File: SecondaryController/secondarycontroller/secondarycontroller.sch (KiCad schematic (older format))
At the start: 11 parts

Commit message: Meh, doesnt work
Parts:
- CF15: footprint (none) -> Capacitor_THT:C_Rect_L41.5mm_W19.0mm_P37.50mm_MKS4; symbol Device:C -> secondarycontroller-rescue:C-Device
- D1, D2: renamed from D?; footprint (none) -> Diode_THT:D_5W_P12.70mm_Horizontal; symbol pspice:DIODE -> secondarycontroller-rescue:DIODE-pspice
- J1: renamed from J?; value Conn_01x03_Female -> Receiver; footprint (none) -> Connector_PinHeader_2.54mm:PinHeader_1x03_P2.54mm_Vertical; symbol Connector:Conn_01x03_Female -> secondarycontroller-rescue:Conn_01x03_Female-Connector
- J3: renamed from J?; value Conn_01x02_Female -> VIN; footprint (none) -> Connector_PinHeader_2.54mm:PinHeader_1x02_P2.54mm_Vertical; symbol Connector:Conn_01x02_Female -> secondarycontroller-rescue:Conn_01x02_Female-Connector
- J4: renamed from J?; footprint (none) -> Connector_PinHeader_2.54mm:PinHeader_1x04_P2.54mm_Vertical; symbol Connector:Conn_01x04_Female -> secondarycontroller-rescue:Conn_01x04_Female-Connector
- J5: renamed from J?; value Conn_01x02_Female -> I2C BUS; footprint (none) -> Connector_PinHeader_2.54mm:PinHeader_1x02_P2.54mm_Vertical; symbol Connector:Conn_01x02_Female -> secondarycontroller-rescue:Conn_01x02_Female-Connector
- SW1: renamed from Calibrate; value SW_Push -> Calibrate; footprint (none) -> Button_Switch_THT:SW_DIP_SPSTx01_Piano_10.8x4.1mm_W7.62mm_P2.54mm; symbol Switch:SW_Push -> secondarycontroller-rescue:SW_Push-Switch
- SW2: renamed from Reset; value SW_Push -> Reset; footprint (none) -> Button_Switch_THT:SW_DIP_SPSTx01_Piano_10.8x4.1mm_W7.62mm_P2.54mm; symbol Switch:SW_Push -> secondarycontroller-rescue:SW_Push-Switch
- U1: renamed from U?; symbol mcu3386:MCU3386 -> secondarycontroller-rescue:MCU3386-mcu3386
- XA1: renamed from XA?; symbol arduino:Arduino_Uno_Shield -> secondarycontroller-rescue:Arduino_Uno_Shield-arduino
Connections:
- wire segments 73 -> 68
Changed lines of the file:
@@
 EESchema Schematic File Version 4
+LIBS:secondarycontroller-cache
 EELAYER 26 0
 EELAYER END
@@
 $EndDescr
 $Comp
-L arduino:Arduino_Uno_Shield XA?
+L secondarycontroller-rescue:Arduino_Uno_Shield-arduino XA1
 U 1 1 5BBE520D
 P 4100 2750
-F 0 "XA?" H 4100 4137 60  0000 C CNN
+F 0 "XA1" H 4100 4137 60  0000 C CNN
 F 1 "Arduino_Uno_Shield" H 4100 4031 60  0000 C CNN
 F 2 "" H 5900 6500 60  0001 C CNN
@@
 $EndComp
 $Comp
-L Connector:Conn_01x02_Female J?
+L secondarycontroller-rescue:Conn_01x02_Female-Connector J3
 U 1 1 5BBE53F0
 P 1900 3600
-F 0 "J?" H 1794 3275 50  0000 C CNN
-F 1 "Conn_01x02_Female" H 1794 3366 50  0000 C CNN
-F 2 "" H 1900 3600 50  0001 C CNN
+F 0 "J3" H 1794 3275 50  0000 C CNN
+F 1 "VIN" H 1794 3366 50  0000 C CNN
+F 2 "Connector_PinHeader_2.54mm:PinHeader_1x02_P2.54mm_Vertical" H 1900 3600 50  0001 C CNN
 F 3 "~" H 1900 3600 50  0001 C CNN
 	1    1900 3600
@@
 	2550 3300 2800 3300
 $Comp
-L Device:C CF15
+L secondarycontroller-rescue:C-Device CF15
 U 1 1 5BBE583A
 P 2400 4300
 F 0 "CF15" V 2148 4300 50  0000 C CNN
 F 1 "C" V 2239 4300 50  0000 C CNN
-F 2 "" H 2438 4150 50  0001 C CNN
+F 2 "Capacitor_THT:C_Rect_L41.5mm_W19.0mm_P37.50mm_MKS4" H 2438 4150 50  0001 C CNN
 F 3 "~" H 2400 4300 50  0001 C CNN
 	1    2400 4300
@@
 $EndComp
 $Comp
-L pspice:DIODE D?
+L secondarycontroller-rescue:DIODE-pspice D2
 U 1 1 5BBE5A38
 P 2550 5100
-F 0 "D?" V 2596 4972 50  0000 R CNN
+F 0 "D2" V 2596 4972 50  0000 R CNN
 F 1 "DIODE" V 2505 4972 50  0000 R CNN
-F 2 "" H 2550 5100 50  0001 C CNN
+F 2 "Diode_THT:D_5W_P12.70mm_Horizontal" H 2550 5100 50  0001 C CNN
 F 3 "~" H 2550 5100 50  0001 C CNN
 	1    2550 5100
@@
 $EndComp
 $Comp
-L Switch:SW_Push Reset
+L secondarycontroller-rescue:SW_Push-Switch SW2
 U 1 1 5BBE645A
 P 4100 4300
-F 0 "Reset" H 4100 4585 50  0000 C CNN
-F 1 "SW_Push" H 4100 4494 50  0000 C CNN
-F 2 "" H 4100 4500 50  0001 C CNN
+F 0 "SW2" H 4100 4585 50  0000 C CNN
+F 1 "Reset" H 4100 4494 50  0000 C CNN
+F 2 "Button_Switch_THT:SW_DIP_SPSTx01_Piano_10.8x4.1mm_W7.62mm_P2.54mm" H 4100 4500 50  0001 C CNN
 F 3 "" H 4100 4500 50  0001 C CNN
 	1    4100 4300
@@
 $EndComp
 $Comp
-L Connector:Conn_01x04_Female J?
+L secondarycontroller-rescue:Conn_01x04_Female-Connector J4
 U 1 1 5BBE6815
 P 6250 1600
-F 0 "J?" H 6278 1576 50  0000 L CNN
+F 0 "J4" H 6278 1576 50  0000 L CNN
 F 1 "APA102C" H 6278 1485 50  0000 L CNN
-F 2 "" H 6250 1600 50  0001 C CNN
+F 2 "Connector_PinHeader_2.54mm:PinHeader_1x04_P2.54mm_Vertical" H 6250 1600 50  0001 C CNN
 F 3 "~" H 6250 1600 50  0001 C CNN
 	1    6250 1600
@@
 $EndComp
 $Comp
-L Switch:SW_Push Calibrate
+L secondarycontroller-rescue:SW_Push-Switch SW1
 U 1 1 5BBE694D
-P 7100 2050
-F 0 "Calibrate" H 7100 2335 50  0000 C CNN
-F 1 "SW_Push" H 7100 2244 50  0000 C CNN
-F 2 "" H 7100 2250 50  0001 C CNN
-F 3 "" H 7100 2250 50  0001 C CNN
-	1    7100 2050
+P 5600 2100
+F 0 "SW1" H 5600 2385 50  0000 C CNN
+F 1 "Calibrate" H 5600 2294 50  0000 C CNN
+F 2 "Button_Switch_THT:SW_DIP_SPSTx01_Piano_10.8x4.1mm_W7.62mm_P2.54mm" H 5600 2300 50  0001 C CNN
+F 3 "" H 5600 2300 50  0001 C CNN
+	1    5600 2100
 	1    0    0    -1
 $EndComp
@@
 Connection ~ 2550 3600
 $Comp
-L mcu3386:MCU3386 U?
+L secondarycontroller-rescue:MCU3386-mcu3386 U1
 U 1 1 5BBE76D9
 P 1300 4750
-F 0 "U?" H 1350 4865 50  0000 C CNN
+F 0 "U1" H 1350 4865 50  0000 C CNN
 F 1 "MCU3386" H 1350 4774 50  0000 C CNN
 F 2 "" H 1300 4750 50  0001 C CNN
@@
 	2550 4300 2550 3600
 $Comp
-L pspice:DIODE D?
+L secondarycontroller-rescue:DIODE-pspice D1
 U 1 1 5BBE875F
 P 2200 5200
-F 0 "D?" H 2200 4935 50  0000 C CNN
+F 0 "D1" H 2200 4935 50  0000 C CNN
 F 1 "DIODE" H 2200 5026 50  0000 C CNN
-F 2 "" H 2200 5200 50  0001 C CNN
+F 2 "Diode_THT:D_5W_P12.70mm_Horizontal" H 2200 5200 50  0001 C CNN
 F 3 "~" H 2200 5200 50  0001 C CNN
 	1    2200 5200
@@
 	1550 4300 2250 4300
 $Comp
-L Connector:Conn_01x03_Female J?
+L secondarycontroller-rescue:Conn_01x03_Female-Connector J1
 U 1 1 5BBEDF33
 P 6200 2300
-F 0 "J?" H 6227 2326 50  0000 L CNN
-F 1 "Conn_01x03_Female" H 6227 2235 50  0000 L CNN
-F 2 "" H 6200 2300 50  0001 C CNN
+F 0 "J1" H 6227 2326 50  0000 L CNN
+F 1 "Receiver" H 6227 2235 50  0000 L CNN
+F 2 "Connector_PinHeader_2.54mm:PinHeader_1x03_P2.54mm_Vertical" H 6200 2300 50  0001 C CNN
 F 3 "~" H 6200 2300 50  0001 C CNN
 	1    6200 2300
@@
 Connection ~ 2900 5400
 Wire Wire Line
-	5400 2100 5800 2100
-Wire Wire Line
-	5800 2100 5800 1950
-Wire Wire Line
-	5800 1950 6900 1950
-Wire Wire Line
-	6900 1950 6900 2050
-Wire Wire Line
-	7300 2050 7300 1400
-Wire Wire Line
-	7300 1400 5850 1400
-Wire Wire Line
-	5850 1400 5850 1500
-Connection ~ 5850 1500
+	5800 2100 5850 2100
+Wire Wire Line
+	5850 2100 5850 2050
 Wire Wire Line
 	5850 1500 5850 2050
 $Comp
-L Connector:Conn_01x02_Female J?
+L secondarycontroller-rescue:Conn_01x02_Female-Connector J5
 U 1 1 5BBF72BA
 P 2300 2100
-F 0 "J?" H 2194 1775 50  0000 C CNN
-F 1 "Conn_01x02_Female" H 2194 1866 50  0000 C CNN
-F 2 "" H 2300 2100 50  0001 C CNN
+F 0 "J5" H 2194 1775 50  0000 C CNN
+F 1 "I2C BUS" H 2194 1866 50  0000 C CNN
+F 2 "Connector_PinHeader_2.54mm:PinHeader_1x02_P2.54mm_Vertical" H 2300 2100 50  0001 C CNN
 F 3 "~" H 2300 2100 50  0001 C CNN
 	1    2300 2100
@@
 Wire Wire Line
 	2500 2100 2800 2100
+Connection ~ 5850 2050
 $EndSCHEMATC

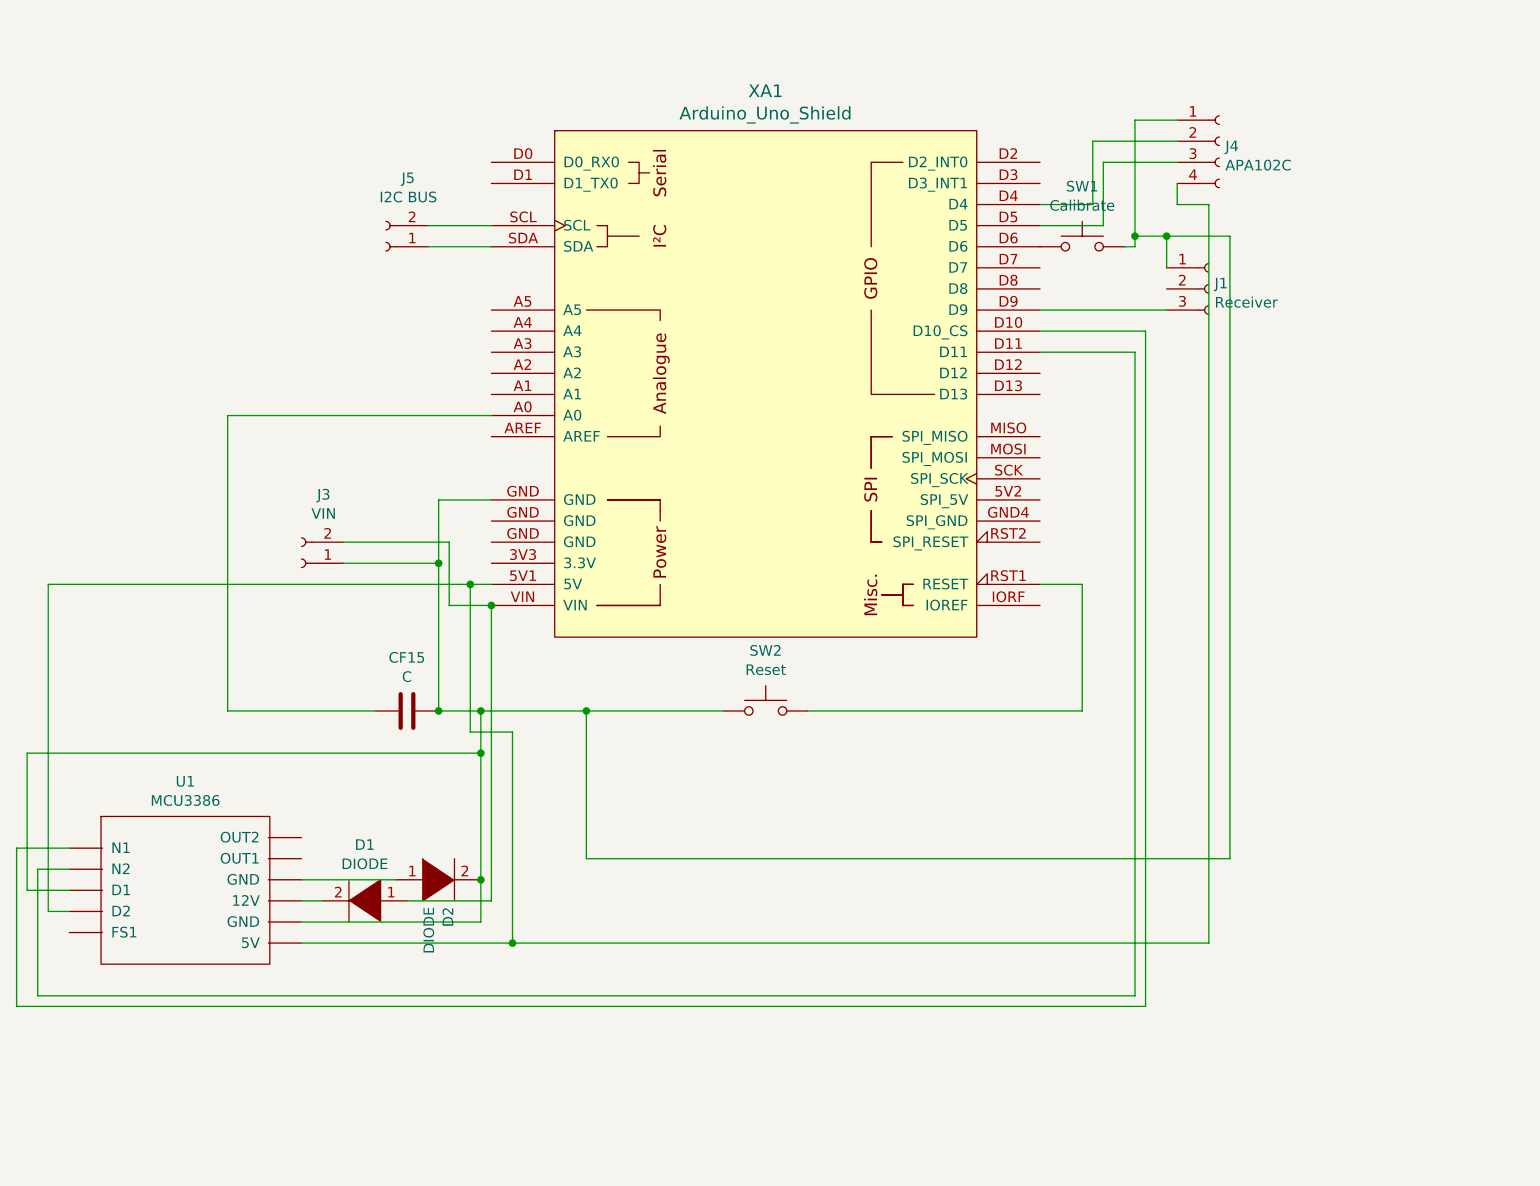
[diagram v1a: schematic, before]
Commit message: Finished PCB Secondary
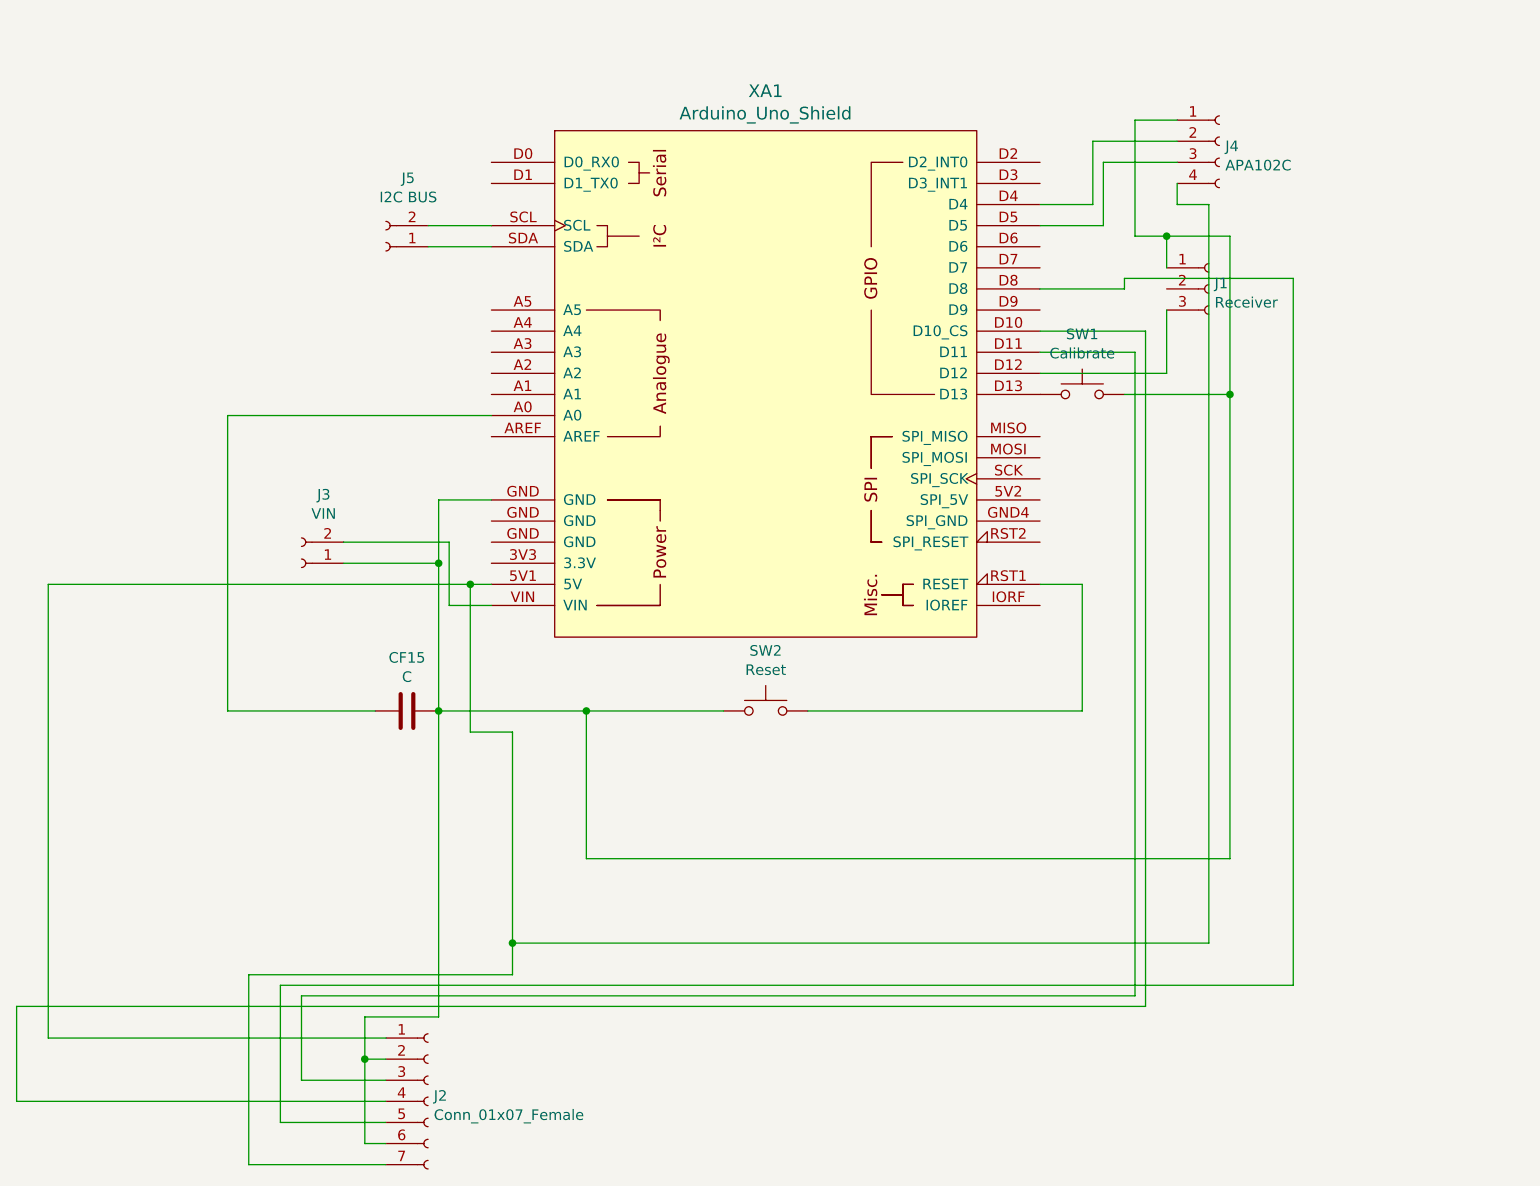
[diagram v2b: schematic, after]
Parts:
- removed D1, D2: DIODE, Diode_THT:D_5W_P12.70mm_Horizontal, symbol secondarycontroller-rescue:DIODE-pspice
- removed U1: MCU3386, symbol secondarycontroller-rescue:MCU3386-mcu3386
- added J2: Conn_01x07_Female, Connector_PinSocket_2.54mm:PinSocket_1x07_P2.54mm_Vertical, symbol Connector:Conn_01x07_Female
- CF15: footprint Capacitor_THT:C_Rect_L41.5mm_W19.0mm_P37.50mm_MKS4 -> Capacitor_THT:C_Rect_L41.5mm_W13.0mm_P37.50mm_MKS4
- SW1, SW2: footprint Button_Switch_THT:SW_DIP_SPSTx01_Piano_10.8x4.1mm_W7.62mm_P2.54mm -> Button_Switch_THT:SW_PUSH_6mm
- XA1: footprint (none) -> Arduino:Arduino_Uno_Shield
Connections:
- net at J4.4 (Pin_4), XA1.5V1 (5V): now also J2.1 (Pin_1), J2.7 (Pin_7)
- net at XA1.D10 (D10_CS): now also J2.4 (Pin_4)
- net at XA1.D11: now also J2.3 (Pin_3)
- net at XA1.D12: now also J1.3 (Pin_3)
- net at XA1.D13: now also SW1.1
- net at XA1.D6: no longer SW1.1
- net at XA1.D8: now also J2.5 (Pin_5)
- net at XA1.D9: no longer J1.3 (Pin_3)
- net at XA1.GND: now also CF15.1, J1.1 (Pin_1), J3.1 (Pin_1), J4.1 (Pin_1), SW1.2, SW2.1, J2.2 (Pin_2), J2.6 (Pin_6)
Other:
- moved on the sheet: SW1
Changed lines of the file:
@@
 F 0 "XA1" H 4100 4137 60  0000 C CNN
 F 1 "Arduino_Uno_Shield" H 4100 4031 60  0000 C CNN
-F 2 "" H 5900 6500 60  0001 C CNN
+F 2 "Arduino:Arduino_Uno_Shield" H 5900 6500 60  0001 C CNN
 F 3 "https://store.arduino.cc/arduino-uno-rev3" H 5900 6500 60  0001 C CNN
 	1    4100 2750
@@
 F 0 "CF15" V 2148 4300 50  0000 C CNN
 F 1 "C" V 2239 4300 50  0000 C CNN
-F 2 "Capacitor_THT:C_Rect_L41.5mm_W19.0mm_P37.50mm_MKS4" H 2438 4150 50  0001 C CNN
+F 2 "Capacitor_THT:C_Rect_L41.5mm_W13.0mm_P37.50mm_MKS4" H 2438 4150 50  0001 C CNN
 F 3 "~" H 2400 4300 50  0001 C CNN
 	1    2400 4300
 	0    1    1    0
-$EndComp
-$Comp
-L secondarycontroller-rescue:DIODE-pspice D2
-U 1 1 5BBE5A38
-P 2550 5100
-F 0 "D2" V 2596 4972 50  0000 R CNN
-F 1 "DIODE" V 2505 4972 50  0000 R CNN
-F 2 "Diode_THT:D_5W_P12.70mm_Horizontal" H 2550 5100 50  0001 C CNN
-F 3 "~" H 2550 5100 50  0001 C CNN
-	1    2550 5100
-	1    0    0    -1
 $EndComp
 $Comp
@@
 F 0 "SW2" H 4100 4585 50  0000 C CNN
 F 1 "Reset" H 4100 4494 50  0000 C CNN
-F 2 "Button_Switch_THT:SW_DIP_SPSTx01_Piano_10.8x4.1mm_W7.62mm_P2.54mm" H 4100 4500 50  0001 C CNN
+F 2 "Button_Switch_THT:SW_PUSH_6mm" H 4100 4500 50  0001 C CNN
 F 3 "" H 4100 4500 50  0001 C CNN
 	1    4100 4300
@@
 L secondarycontroller-rescue:SW_Push-Switch SW1
 U 1 1 5BBE694D
-P 5600 2100
-F 0 "SW1" H 5600 2385 50  0000 C CNN
-F 1 "Calibrate" H 5600 2294 50  0000 C CNN
-F 2 "Button_Switch_THT:SW_DIP_SPSTx01_Piano_10.8x4.1mm_W7.62mm_P2.54mm" H 5600 2300 50  0001 C CNN
-F 3 "" H 5600 2300 50  0001 C CNN
-	1    5600 2100
+P 5600 2800
+F 0 "SW1" H 5600 3085 50  0000 C CNN
+F 1 "Calibrate" H 5600 2994 50  0000 C CNN
+F 2 "Button_Switch_THT:SW_PUSH_6mm" H 5600 3000 50  0001 C CNN
+F 3 "" H 5600 3000 50  0001 C CNN
+	1    5600 2800
 	1    0    0    -1
 $EndComp
@@
 	3900 4300 3250 4300
 Connection ~ 2550 3600
-$Comp
-L secondarycontroller-rescue:MCU3386-mcu3386 U1
-U 1 1 5BBE76D9
-P 1300 4750
-F 0 "U1" H 1350 4865 50  0000 C CNN
-F 1 "MCU3386" H 1350 4774 50  0000 C CNN
-F 2 "" H 1300 4750 50  0001 C CNN
-F 3 "" H 1300 4750 50  0001 C CNN
-	1    1300 4750
-	1    0    0    -1
-$EndComp
 Wire Wire Line
 	2550 4300 2550 3600
-$Comp
-L secondarycontroller-rescue:DIODE-pspice D1
-U 1 1 5BBE875F
-P 2200 5200
-F 0 "D1" H 2200 4935 50  0000 C CNN
-F 1 "DIODE" H 2200 5026 50  0000 C CNN
-F 2 "Diode_THT:D_5W_P12.70mm_Horizontal" H 2200 5200 50  0001 C CNN
-F 3 "~" H 2200 5200 50  0001 C CNN
-	1    2200 5200
-	-1   0    0    1
-$EndComp
-Wire Wire Line
-	1900 5200 2000 5200
-Wire Wire Line
-	1900 5100 2350 5100
-Wire Wire Line
-	2750 4300 2750 4500
-Connection ~ 2750 4300
-Wire Wire Line
-	2750 4300 2550 4300
-Wire Wire Line
-	2400 5200 2800 5200
-Connection ~ 2800 3800
-Wire Wire Line
-	2800 3800 2800 5200
 Wire Wire Line
 	2800 3700 2700 3700
@@
 Wire Wire Line
 	2900 4400 2900 5400
-Wire Wire Line
-	2900 5400 1900 5400
-Wire Wire Line
-	2750 5100 2750 5300
-Wire Wire Line
-	2750 5300 1900 5300
-Connection ~ 2750 5100
-Wire Wire Line
-	800  5150 600  5150
-Wire Wire Line
-	600  5150 600  4500
-Wire Wire Line
-	600  4500 2750 4500
-Connection ~ 2750 4500
-Wire Wire Line
-	2750 4500 2750 5100
-Wire Wire Line
-	800  5250 700  5250
-Wire Wire Line
-	700  5250 700  3700
 Wire Wire Line
 	700  3700 2700 3700
 Connection ~ 2700 3700
 Wire Wire Line
-	800  5050 650  5050
-Wire Wire Line
-	650  5050 650  5650
-Wire Wire Line
-	650  5650 5850 5650
-Wire Wire Line
 	5850 5650 5850 2600
 Wire Wire Line
@@
 	5900 5700 550  5700
 Wire Wire Line
-	550  5700 550  4950
-Wire Wire Line
-	550  4950 800  4950
+	550  5700 550  6150
+Wire Wire Line
+	550  6150 2300 6150
 Connection ~ 2550 4300
 Wire Wire Line
@@
 $EndComp
 Wire Wire Line
-	6000 2400 5400 2400
-Wire Wire Line
 	6000 2200 6000 2050
 Wire Wire Line
 	6000 2050 6300 2050
 Wire Wire Line
-	6300 2050 6300 5000
+	6300 2050 6300 2800
 Wire Wire Line
 	6300 5000 3250 5000
@@
 Connection ~ 3250 4300
 Wire Wire Line
-	3250 4300 2750 4300
-Wire Wire Line
-	5400 1900 5650 1900
-Wire Wire Line
-	5650 1900 5650 1600
-Wire Wire Line
 	5650 1600 6050 1600
 Wire Wire Line
 	5400 2000 5700 2000
-Wire Wire Line
-	5700 2000 5700 1700
-Wire Wire Line
-	5700 1700 6050 1700
 Wire Wire Line
 	6050 1500 5850 1500
@@
 Wire Wire Line
 	6200 5400 2900 5400
-Connection ~ 2900 5400
-Wire Wire Line
-	5800 2100 5850 2100
-Wire Wire Line
-	5850 2100 5850 2050
 Wire Wire Line
 	5850 1500 5850 2050
@@
 Wire Wire Line
 	2500 2100 2800 2100
-Connection ~ 5850 2050
+$Comp
+L Connector:Conn_01x07_Female J2
+U 1 1 5BCA6134
+P 2500 6150
+F 0 "J2" H 2527 6176 50  0000 L CNN
+F 1 "Conn_01x07_Female" H 2527 6085 50  0000 L CNN
+F 2 "Connector_PinSocket_2.54mm:PinSocket_1x07_P2.54mm_Vertical" H 2500 6150 50  0001 C CNN
+F 3 "~" H 2500 6150 50  0001 C CNN
+	1    2500 6150
+	1    0    0    -1
+$EndComp
+Wire Wire Line
+	700  3700 700  5850
+Wire Wire Line
+	700  5850 2300 5850
+Wire Wire Line
+	5850 5650 1900 5650
+Wire Wire Line
+	1900 5650 1900 6050
+Wire Wire Line
+	1900 6050 2300 6050
+Wire Wire Line
+	2900 5400 2900 5550
+Wire Wire Line
+	2900 5550 1650 5550
+Wire Wire Line
+	1650 5550 1650 6450
+Wire Wire Line
+	1650 6450 2300 6450
+Connection ~ 2900 5400
+Wire Wire Line
+	2300 6250 1800 6250
+Wire Wire Line
+	1800 6250 1800 5600
+Wire Wire Line
+	1800 5600 6600 5600
+Wire Wire Line
+	6600 5600 6600 2250
+Wire Wire Line
+	6600 2250 5800 2250
+Wire Wire Line
+	5800 2300 5400 2300
+Wire Wire Line
+	2550 4300 3250 4300
+Wire Wire Line
+	2550 5750 2200 5750
+Wire Wire Line
+	2200 5750 2200 5950
+Wire Wire Line
+	2200 5950 2300 5950
+Wire Wire Line
+	2200 5950 2200 6350
+Wire Wire Line
+	2200 6350 2300 6350
+Connection ~ 2200 5950
+Wire Wire Line
+	2550 4300 2550 5750
+Wire Wire Line
+	5800 2250 5800 2300
+Wire Wire Line
+	5800 2800 6300 2800
+Connection ~ 6300 2800
+Wire Wire Line
+	6300 2800 6300 5000
+Wire Wire Line
+	6000 2400 6000 2700
+Wire Wire Line
+	6000 2700 5400 2700
+Wire Wire Line
+	5400 1900 5650 1900
+Wire Wire Line
+	5650 1600 5650 1900
+Wire Wire Line
+	5700 1700 5700 2000
+Wire Wire Line
+	5700 1700 6050 1700
 $EndSCHEMATC
